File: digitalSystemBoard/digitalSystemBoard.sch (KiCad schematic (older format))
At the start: 29 parts, among them J1 Barrel_Jack, J10 BCD_1, J13 Conn_02x03_Odd_Even, J2 OUTPUT_HEADER, J3 7_LED_IN_2, J4 7_LED_IN_1, J5 INPUT_HEADER, J6 SN7447, J7 SN7447, J9 BCD_2, Q1 MJD122T4G, SW1 SW_SPDT, SW2 ButtonFirst, SW3 ButtonFirst, U1 LM317, U15 KCSA02-105, U16 KCSA02-105, U2 Potentiometer

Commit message: Upload PCB footprint
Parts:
- J1: footprint Connector_BarrelJack:BarrelJack_Horizontal -> footprints:BARREL_JACK
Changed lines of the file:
@@
 F 0 "J1" H 907 1491 50  0000 C CNN
 F 1 "Barrel_Jack" H 907 1400 50  0000 C CNN
-F 2 "Connector_BarrelJack:BarrelJack_Horizontal" H 900 1126 50  0001 C CNN
+F 2 "footprints:BARREL_JACK" H 900 1126 50  0001 C CNN
 F 3 "~" H 900 1126 50  0001 C CNN
 	1    850  1166

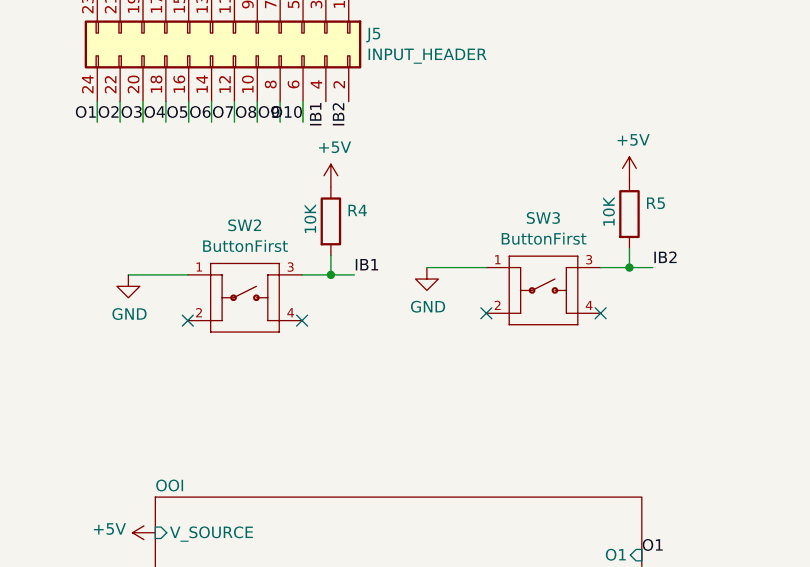
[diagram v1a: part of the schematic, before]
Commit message: Upload after error
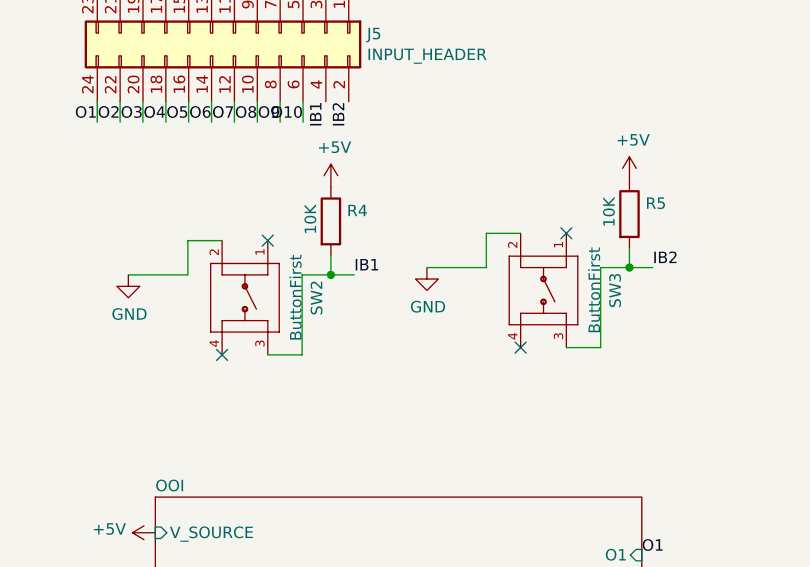
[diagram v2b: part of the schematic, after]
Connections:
- net GND: now also SW2.2, SW3.2; no longer SW2.1, SW3.1
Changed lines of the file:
@@
 F 6 "Compliant" H 1872 4446 50  0001 L BNN "Field6"
 	1    1872 4446
-	1    0    0    -1
+	0    1    1    0
 $EndComp
 Text Label 2350 4346 0    50   ~ 0
@@
 	1    0    0    -1
 $EndComp
-NoConn ~ 2122 4546
-NoConn ~ 1622 4546
+NoConn ~ 1772 4696
+NoConn ~ 1972 4196
 $Comp
 L power:GND #PWR0101
@@
 F 6 "Compliant" H 3178 4414 50  0001 L BNN "Field6"
 	1    3178 4414
-	1    0    0    -1
+	0    1    1    0
 $EndComp
 Connection ~ 3554 4314
@@
 	1    0    0    -1
 $EndComp
-NoConn ~ 3428 4514
-NoConn ~ 2928 4514
+NoConn ~ 3278 4164
+NoConn ~ 3078 4664
 $Comp
 L power:+5V #PWR0102
@@
 Text Label 2026 3088 2    50   ~ 0
 O9
+Wire Wire Line
+	1772 4196 1622 4196
+Wire Wire Line
+	1622 4196 1622 4346
+Wire Wire Line
+	2122 4346 2122 4696
+Wire Wire Line
+	2122 4696 1972 4696
+Wire Wire Line
+	3078 4164 2928 4164
+Wire Wire Line
+	2928 4164 2928 4314
+Wire Wire Line
+	3428 4314 3428 4664
+Wire Wire Line
+	3428 4664 3278 4664
 $EndSCHEMATC
